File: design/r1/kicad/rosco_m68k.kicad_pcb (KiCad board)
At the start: 4 copper layers, 160 x 100 mm, 74 parts, among them IC1 MC68010P10, IC2 ATF16V8BQL-15PU, IC3 7493N, IC4 MC68901P, IC5 ATF16V8BQL, IC6 74174N, IC7 7404N, IC8 555N, IC9 74LS01N, Q1 3.6864MHz, Q2 8MHz, U1 AT28C64B-15PU, U2 AT28C64B-15PU, U3 AS6C4008-55PCN, U4 AS6C4008-55PCN

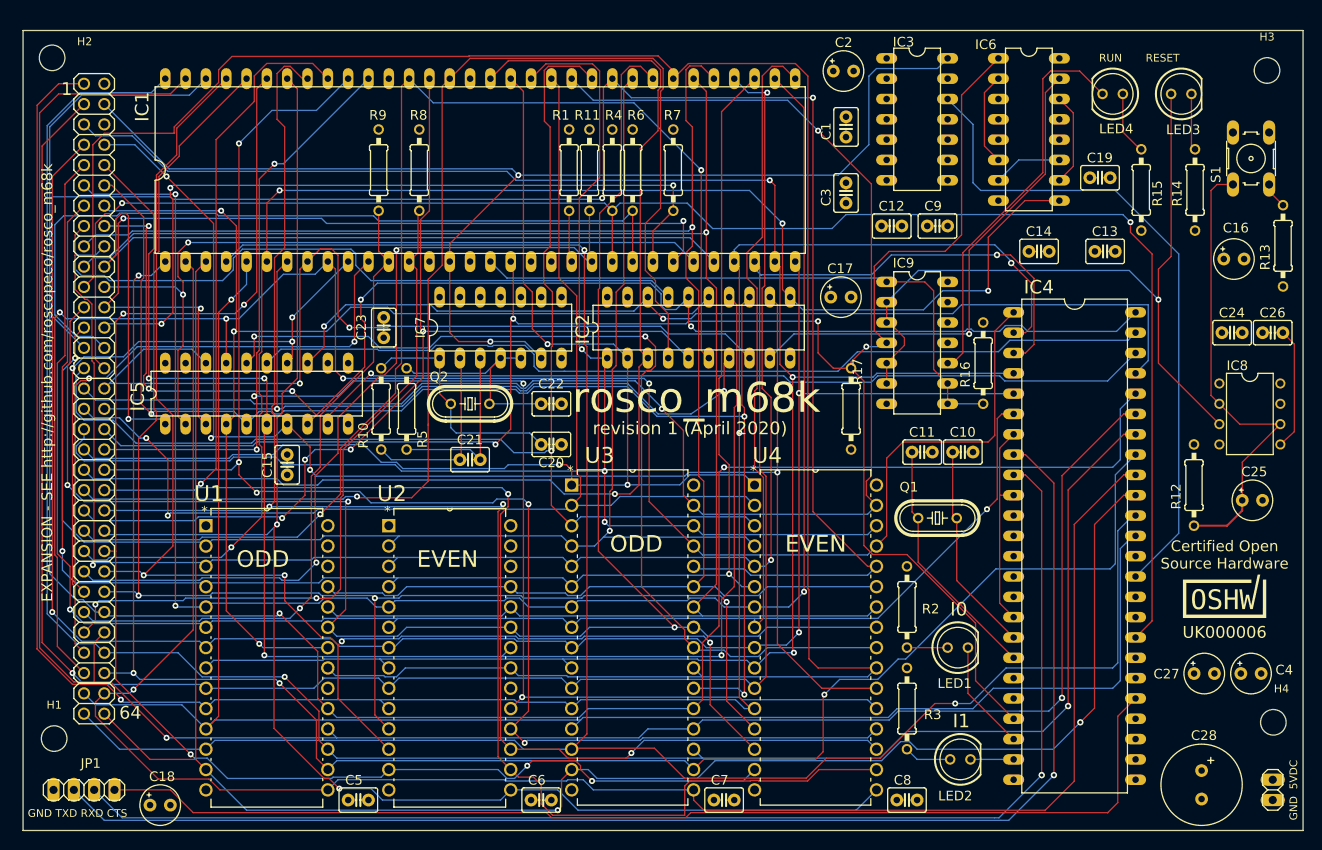
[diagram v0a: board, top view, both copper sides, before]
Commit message: Design complete
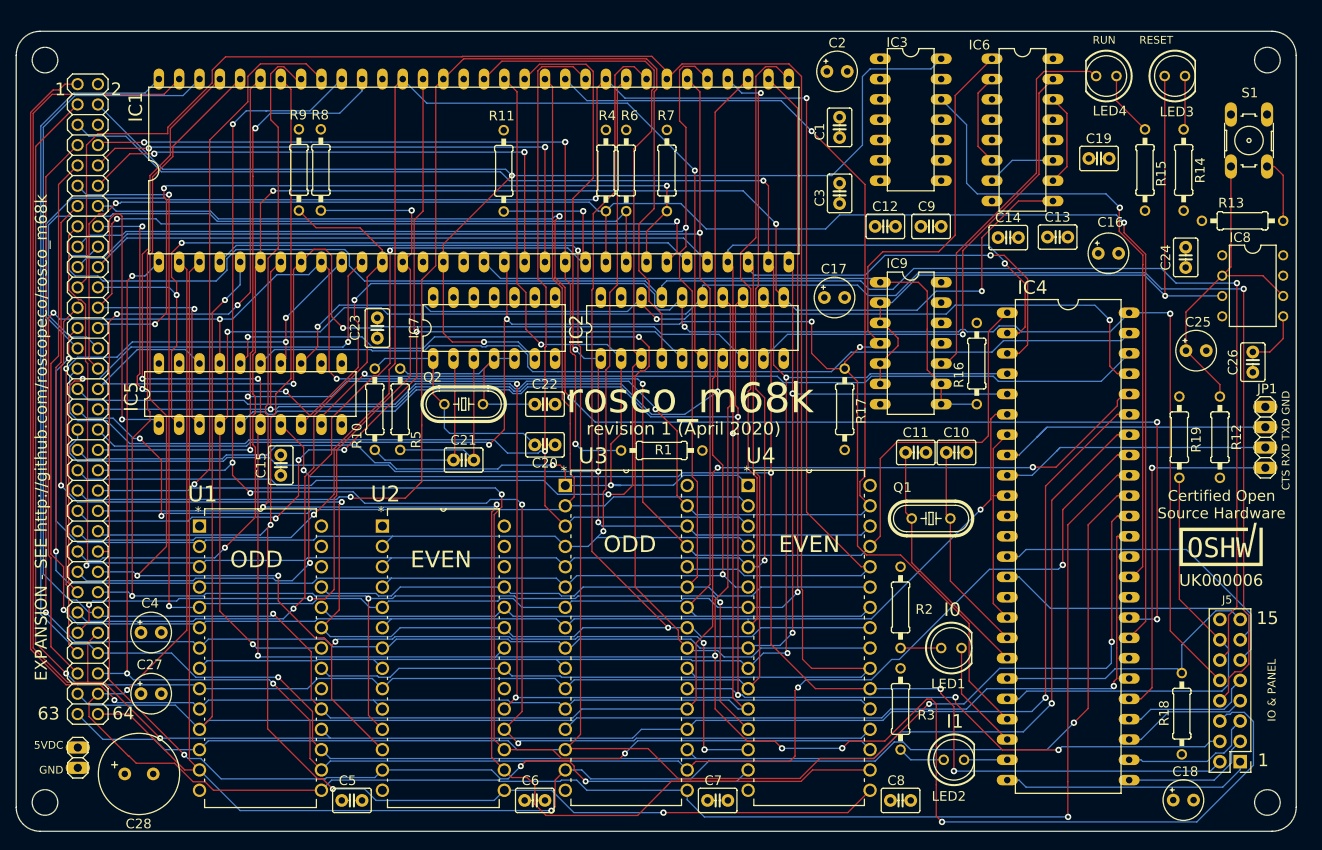
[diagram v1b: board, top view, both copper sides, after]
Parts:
- added J5: GPIO-PANEL, Connector_PinHeader_2.54mm:PinHeader_2x08_P2.54mm_Vertical, F.Cu at (220.9, 146.4)
- added R18: 4K7, rosco_m68k:0207_10, F.Cu at (213.6, 140.4)
- added R19: 4K7, rosco_m68k:0207_10, F.Cu at (213.3, 105.8)
- added REF**: KiCad-Logo2_5mm_SilkScreen, Symbol:KiCad-Logo2_5mm_SilkScreen, B.Cu at (117.0, 70.2)
- moved JP1 154.1 mm to (224.0, 105.9), turned to 270 degrees
- moved JP2 149.4 mm to (75.6, 145.9)
- moved C4 137.6 mm to (84.8, 130.2)
- moved C28 132.8 mm to (83.2, 147.9), turned to 0 degrees
- moved C27 131.7 mm to (84.8, 137.9)
- moved C18 127.9 mm to (213.8, 151.2)
- moved R1 36.9 mm to (148.6, 107.5), turned to 180 degrees
- moved C25 20.0 mm to (215.4, 95.0)
- moved IC8 16.0 mm to (222.5, 86.9)
- moved C16 15.7 mm to (204.4, 82.9)
- moved R8 12.3 mm to (106.0, 72.4)
- moved C24 11.1 mm to (214.1, 83.4), turned to 90 degrees
- moved R11 10.7 mm to (128.8, 72.5)
- moved H4 10.0 mm to (224.3, 151.5)
- moved R9 9.97 mm to (103.2, 72.4)
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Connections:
- IC1 pad 19: Net-(IC1-Pad19) -> VMA
- IC1 pad 20: Net-(IC1-Pad20) -> E
- IC1 pad 21: Net-(IC1-Pad21) -> VPA
- IC4 pad 13: Net-(IC4-Pad13) -> TAO
- IC4 pad 14: Net-(IC4-Pad14) -> TBO
- IC4 pad 19: GND -> TAI
- IC4 pad 20: GND -> TBI
- IC4 pad 24: Net-(IC4-Pad24) -> GPIO1
- IC4 pad 25: Net-(IC4-Pad25) -> GPIO2
- IC4 pad 26: Net-(IC4-Pad26) -> GPIO3
- IC4 pad 27: Net-(IC4-Pad27) -> GPIO4
- IC4 pad 28: Net-(IC4-Pad28) -> GPIO5
- IC4 pad 33: Net-(IC4-Pad33) -> IEO
- JP3 pad 10: EVENROMSEL -> E
- JP3 pad 12: ODDRAMSEL -> VMA
- JP3 pad 14: ODDROMSEL -> IEO
- JP3 pad 8: EVENRAMSEL -> VPA
- R1 pad 1: Net-(IC1-Pad21) -> VCC
- R1 pad 2: VCC -> VPA
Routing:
- net IEO: track 0.00 -> 185.9 mm, vias 0 -> 4
- net /MC68901_Decoder/UARTTX: track 169.4 -> 38.7 mm, vias 1 -> 0
- net /MC68901_Decoder/UARTRX: track 161.9 -> 37.5 mm, vias 1 -> 0
- net EXPSEL: track 86.4 -> 210.3 mm, vias 0 -> 1
- net VPA: track 0.00 -> 103.4 mm, vias 0 -> 3
- net Net-(IC4-Pad29): track 141.6 -> 45.1 mm, vias 0 -> 1
- net ODDROMSEL: track 142.6 -> 237.2 mm
- net EVENROMSEL: track 183.6 -> 277.2 mm, vias 4 -> 7
- net E: track 0.00 -> 71.6 mm, vias 0 -> 2
- net VMA: track 0.00 -> 68.8 mm, vias 0 -> 2
- net TBI: track 0.00 -> 56.8 mm
- net IOSEL: track 173.6 -> 227.2 mm, vias 5 -> 6
- net TAO: track 0.00 -> 40.5 mm
- net TBO: track 0.00 -> 35.7 mm
- net TAI: track 0.00 -> 35.6 mm
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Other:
- outline, holes or cut-outs redrawn
- board text added: "15"
- board text added: "2"
- board text added: "5VDC GND"
- board text added: "63"
- board text added: "CTS RXD TXD GND"
- board text added: "IO & PANEL"
- board text removed: "GND 5VDC"
- board text removed: "GND TXD RXD CTS"
